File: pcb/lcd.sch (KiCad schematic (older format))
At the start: 36 parts, among them J500 FPC_18P_1.0MM, Q500 IRLML6402, U100 MCIMX7S5EVM08SC, U500 XC2C32A, U501 ADP5075, U502 LM324

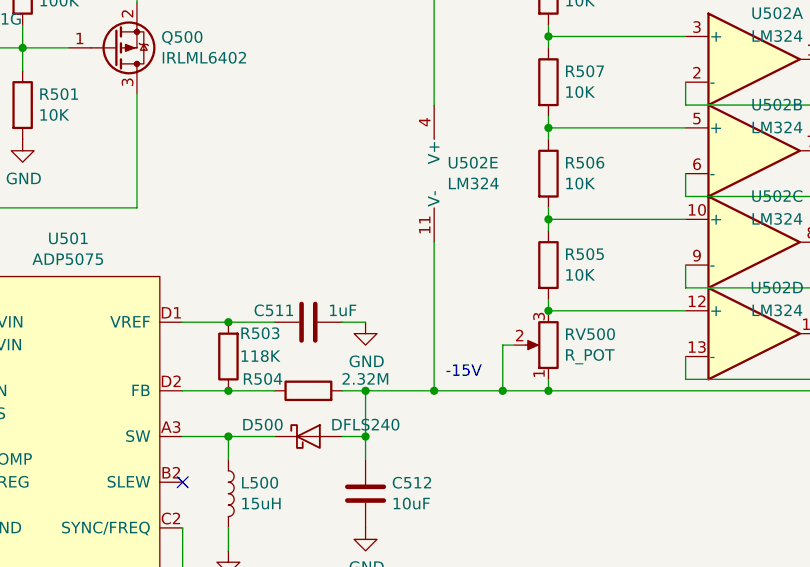
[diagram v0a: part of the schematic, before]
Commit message: pcb: working on sch
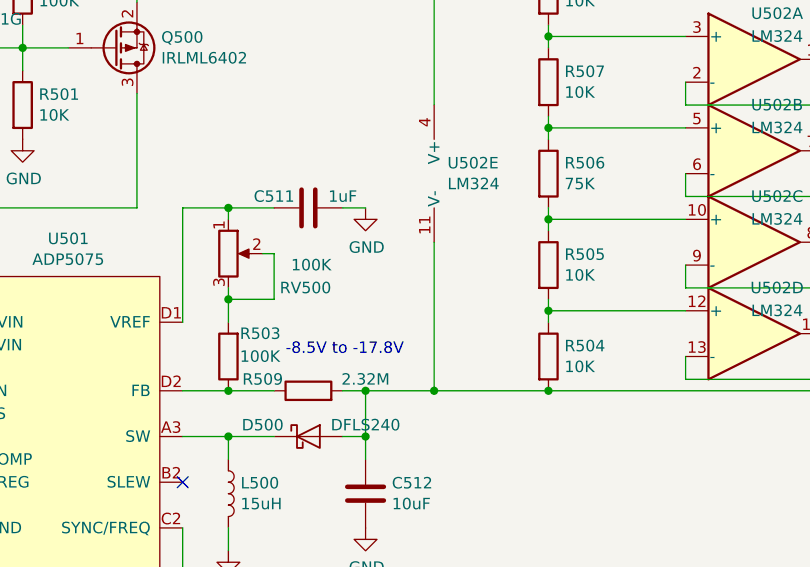
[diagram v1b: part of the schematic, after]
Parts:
- added R504: 10K, symbol Device:R
- R503: value 118K -> 100K
- R506: value 10K -> 75K
- RV500: value R_POT -> 100K
- renumbered R504 to R509
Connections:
- wire segments 199 -> 203
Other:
- note added: "-8.5V to -17.8V"
- note removed: "-15V"
- moved on the sheet: C511, RV500
